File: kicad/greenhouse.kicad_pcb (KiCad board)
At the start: 2 copper layers, 23 parts, among them J1 Screw_Terminal_01x02, J2 moisture sensor, J3 fan, J4 DHT11, J5 Conn_01x04, J6 Barrel_Jack_Switch, Q1 IRLZ44N, U1 ESP-12F, U2 LM2596S-3.3

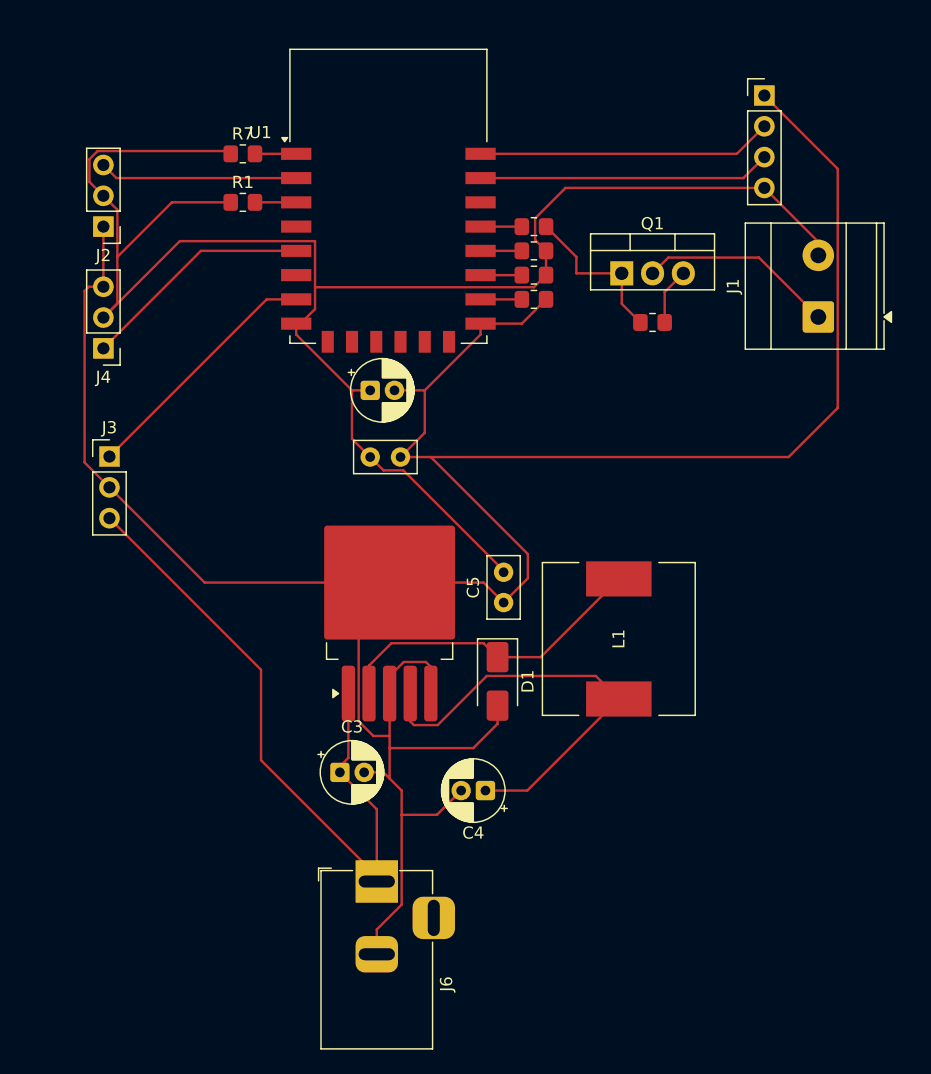
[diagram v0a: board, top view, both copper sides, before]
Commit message: 123
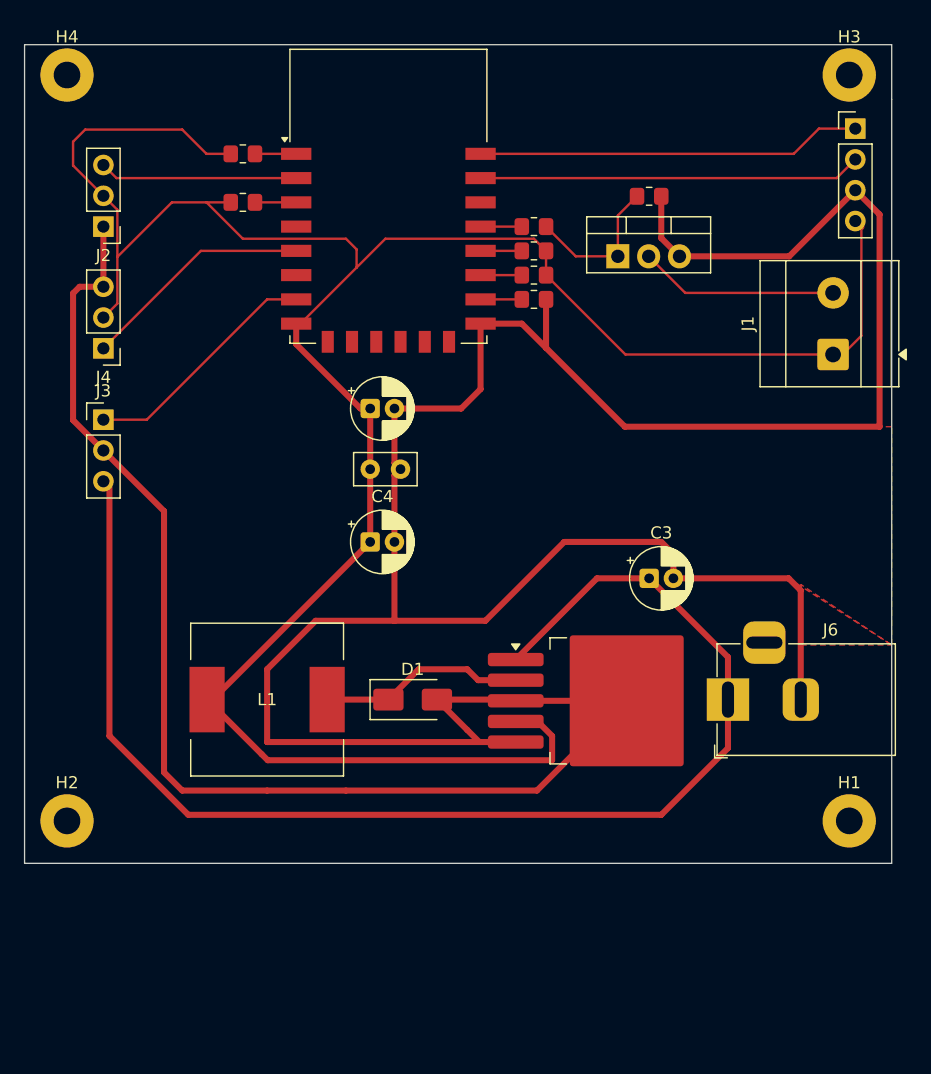
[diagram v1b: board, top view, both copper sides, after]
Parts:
- removed C5: 100nF, Capacitor_THT:C_Disc_D5.0mm_W2.5mm_P2.50mm
- added H1: MountingHole, MountingHole:MountingHole_2.2mm_M2_Pad, F.Cu at (155.0, 138.0)
- added H2: MountingHole, MountingHole:MountingHole_2.2mm_M2_Pad, F.Cu at (90.5, 138.0)
- added H3: MountingHole, MountingHole:MountingHole_2.2mm_M2_Pad, F.Cu at (155.0, 76.5)
- added H4: MountingHole, MountingHole:MountingHole_2.2mm_M2_Pad, F.Cu at (90.5, 76.5)
- moved J6 32.6 mm to (145.0, 128.0), turned to 180 degrees
- moved C3 30.1 mm to (138.5, 118.0)
- moved L1 29.4 mm to (107.0, 128.0), turned to 180 degrees
- moved C4 22.6 mm to (115.5, 115.0), turned to 0 degrees
- moved U2 19.8 mm to (135.2, 128.1), turned to 0 degrees
- moved R3 10.4 mm to (138.5, 86.5)
- moved J5 7.98 mm to (155.5, 80.9)
- moved D1 7.16 mm to (119.0, 128.0), turned to 0 degrees
- moved J1 3.33 mm to (153.7, 99.5)
- moved J3 3.08 mm to (93.5, 104.9)
- moved C1 1.50 mm to (115.5, 104.0)
- moved Q1 1.44 mm to (135.9, 91.5)
- moved C2 1.00 mm to (115.5, 109.0)
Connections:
- J1 pad 1: Net-(J1-Pin_1) -> +3.3V
- J1 pad 2: +3.3V -> Net-(J1-Pin_2)
- J5 pad 1: GND -> Net-(J5-Pin_1)
- J5 pad 3: Net-(J5-Pin_3) -> GND
- Q1 pad 2: Net-(J1-Pin_1) -> Net-(J1-Pin_2)
- U1 pad 21: Net-(J5-Pin_3) -> Net-(J5-Pin_2)
- U1 pad 22: Net-(J5-Pin_2) -> Net-(J5-Pin_1)
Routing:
- net GND: track 234.7 -> 316.6 mm
- net +12V: track 56.1 -> 107.6 mm
- net Net-(J5-Pin_1): track 0.00 -> 31.8 mm
- net Net-(J5-Pin_3): track 24.1 -> 0.00 mm
- net +3.3V: track 184.2 -> 200.9 mm
- net Net-(J1-Pin_2): track 0.00 -> 16.5 mm
- net Net-(J1-Pin_1): track 16.2 -> 0.00 mm
- net Net-(D1-K): track 26.8 -> 17.0 mm
- net Net-(J5-Pin_2): track 24.3 -> 31.5 mm
- net gpio4: track 13.8 -> 12.6 mm
- net Net-(J3-Pin_1): track 20.8 -> 20.0 mm
- added copper zone on F.Cu, net GND
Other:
- board outline added: 71.5 x 67.5 mm
